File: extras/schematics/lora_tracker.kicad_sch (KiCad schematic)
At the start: 18 parts, among them J1 Conn_Coaxial, J2 Conn_01x10_Female, J3 Conn_01x12_Female, J4 Conn_01x03_Female, U1 ESP32, U2 E22-400M30S, U3 Ai-Thinker-Ra-01

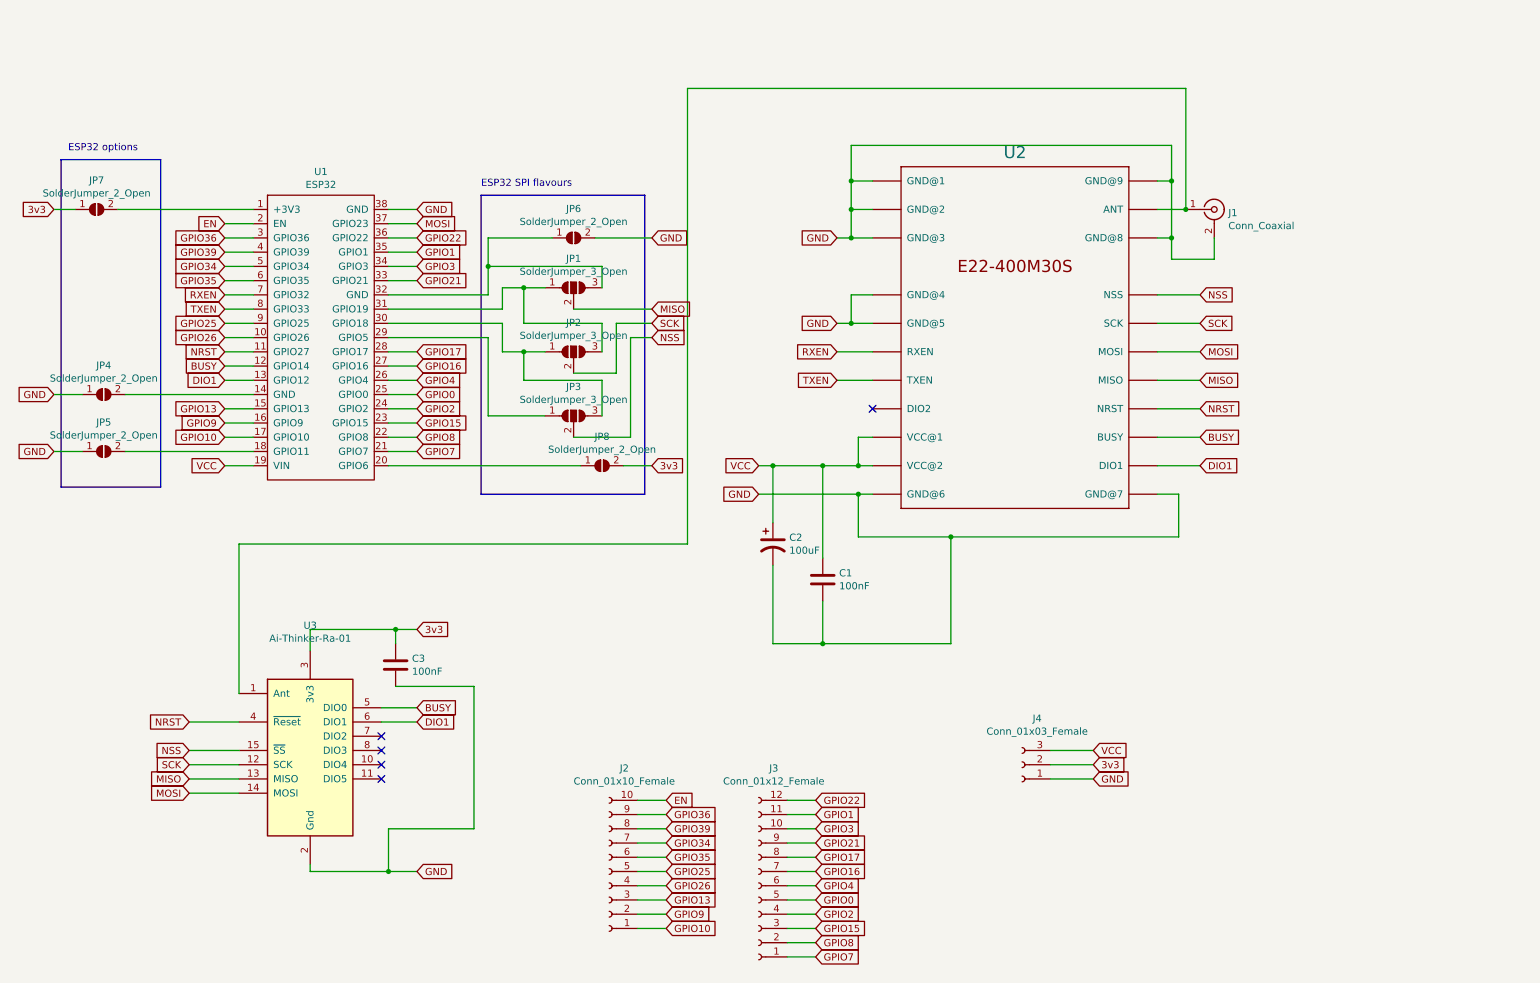
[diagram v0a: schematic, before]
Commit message: Updates
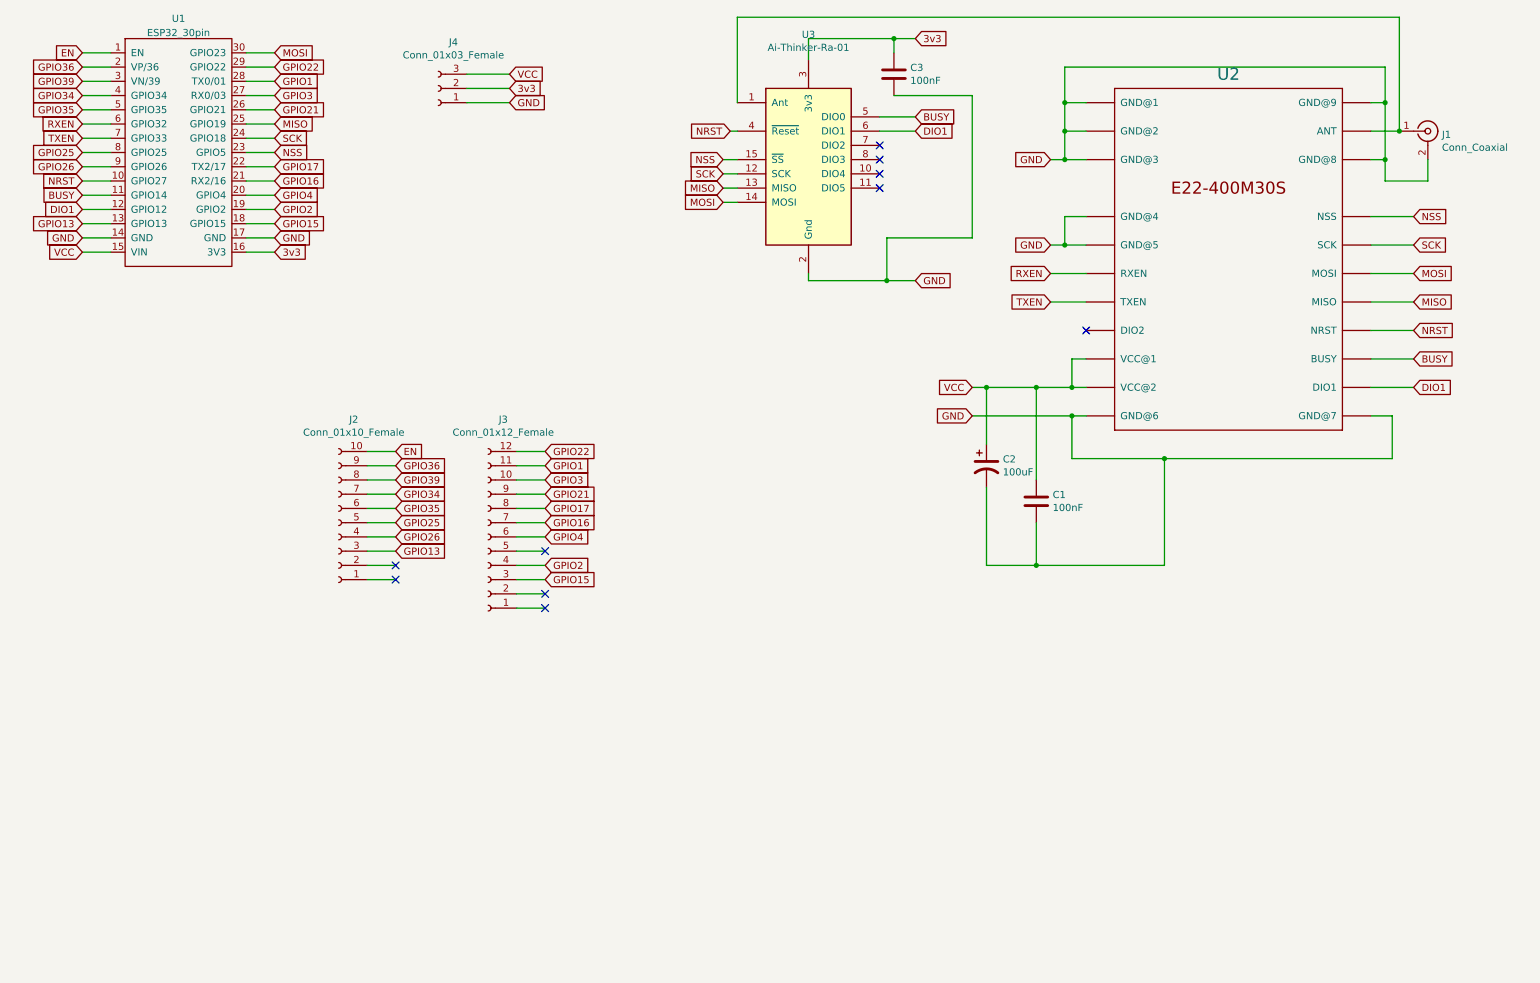
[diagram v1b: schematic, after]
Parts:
- removed JP1, JP2, JP3: SolderJumper_3_Open, Jumper:SolderJumper-3_P1.3mm_Open_Pad1.0x1.5mm, symbol lora_tracker-rescue:SolderJumper_3_Open-Jumper
- removed JP4, JP5, JP6, JP7, JP8: SolderJumper_2_Open, Jumper:SolderJumper-2_P1.3mm_Open_Pad1.0x1.5mm, symbol Jumper:SolderJumper_2_Open
- removed U1: ESP32, lora_tracker:esp32-devkit-wide, symbol lora_tracker:ESP32
- added U1: ESP32_30pin, lora_tracker:esp32-devkit-wide_copy, symbol lora_tracker:ESP32_30pin
- C1, C3: footprint Capacitor_SMD:C_0603_1608Metric_Pad1.05x0.95mm_HandSolder -> Capacitor_SMD:C_0603_1608Metric_Pad1.08x0.95mm_HandSolder
- J1: footprint Connector_Coaxial:SMA_Samtec_SMA-J-P-H-ST-EM1_EdgeMount -> Connector_Coaxial:SMA_Samtec_SMA-J-P-X-ST-EM1_EdgeMount
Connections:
- net 3v3: now also U1.16 (3V3)
- net BUSY: now also U1.11 (GPIO14)
- net DIO1: now also U1.12 (GPIO12)
- net EN: now also U1.1 (EN)
- net GND: now also U1.14 (GND), U1.17 (GND)
- net GPIO1: now also U1.28 (TX0/01)
- net GPIO13: now also U1.13 (GPIO13)
- net GPIO15: now also U1.18 (GPIO15)
- net GPIO16: now also U1.21 (RX2/16)
- net GPIO17: now also U1.22 (TX2/17)
- net GPIO2: now also U1.19 (GPIO2)
- net GPIO21: now also U1.26 (GPIO21)
- net GPIO22: now also U1.29 (GPIO22)
- net GPIO25: now also U1.8 (GPIO25)
- net GPIO26: now also U1.9 (GPIO26)
- net GPIO3: now also U1.27 (RX0/03)
- net GPIO34: now also U1.4 (GPIO34)
- net GPIO35: now also U1.5 (GPIO35)
- net GPIO36: now also U1.2 (VP/36)
- net GPIO39: now also U1.3 (VN/39)
- net GPIO4: now also U1.20 (GPIO4)
- net MISO: now also U1.25 (GPIO19)
- net MOSI: now also U1.30 (GPIO23)
- net NRST: now also U1.10 (GPIO27)
- net NSS: now also U1.23 (GPIO5)
- net RXEN: now also U1.6 (GPIO32)
- net SCK: now also U1.24 (GPIO18)
- net TXEN: now also U1.7 (GPIO33)
- net VCC: now also U1.15 (VIN)
- net GPIO0: no longer names the net of J3.5 (Pin_5)
- net GPIO10: no longer names the net of J2.1 (Pin_1)
- net GPIO7: no longer names the net of J3.1 (Pin_1)
- net GPIO8: no longer names the net of J3.2 (Pin_2)
- net GPIO9: no longer names the net of J2.2 (Pin_2)
- no-connect marks 5 -> 10
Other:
- note removed: "ESP32 SPI flavours"
- note removed: "ESP32 options"
- moved on the sheet: C1, C2, C3, J1, J2, J3, J4, U2, U3

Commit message: Update schematics
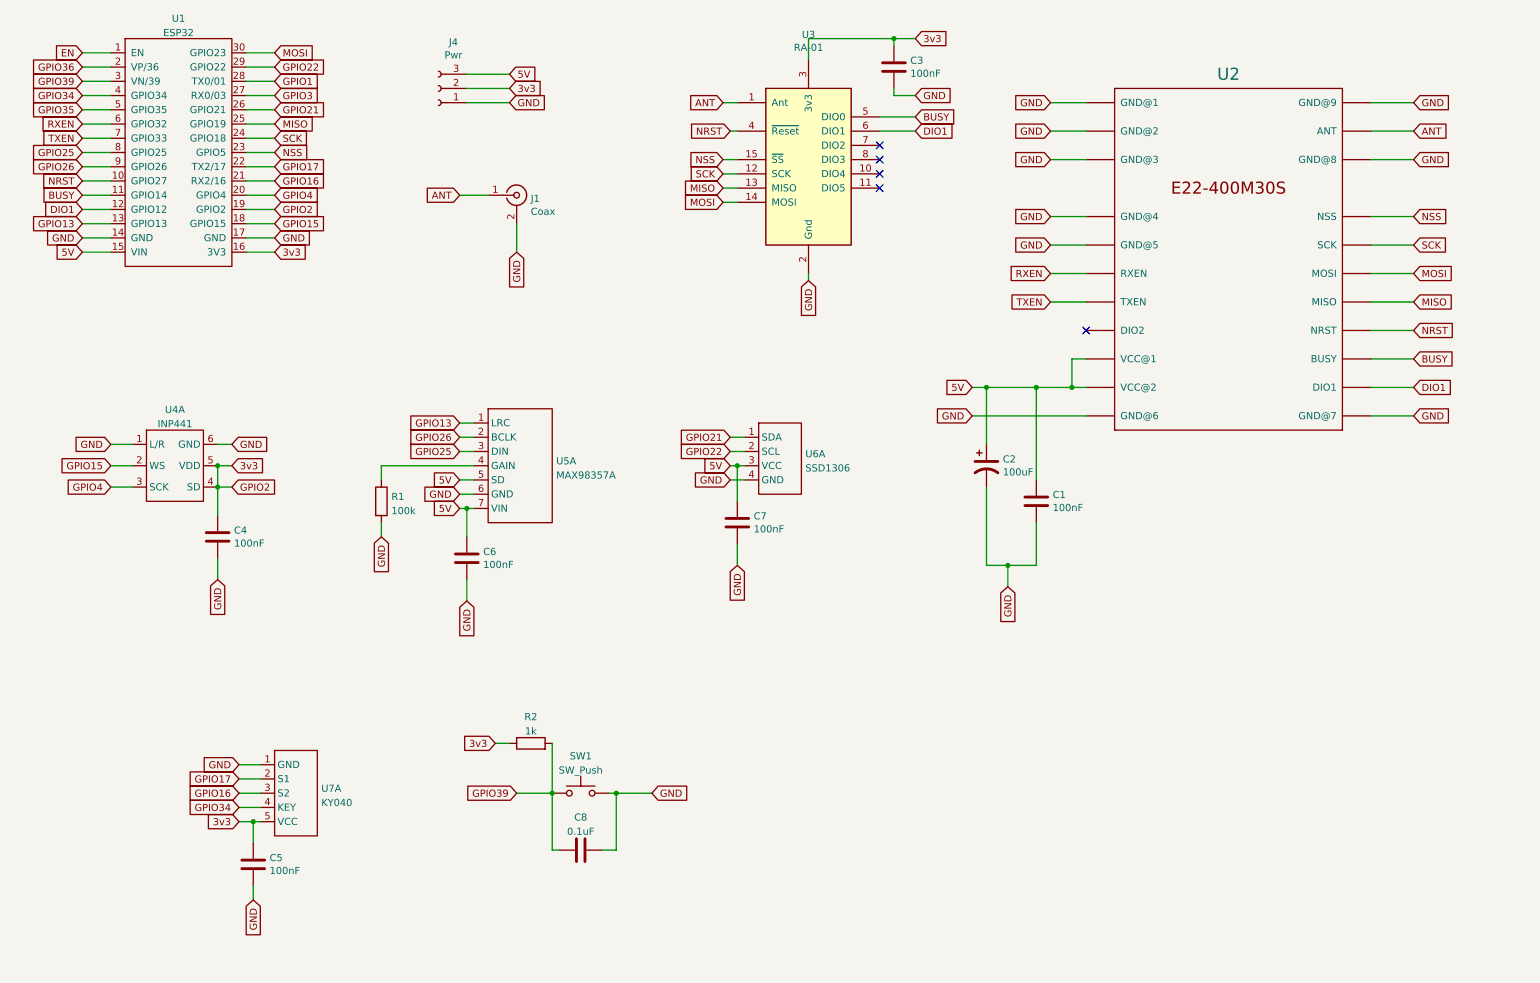
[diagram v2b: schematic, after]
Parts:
- removed J2: Conn_01x10_Female, Connector_PinSocket_2.54mm:PinSocket_1x10_P2.54mm_Vertical, symbol Connector:Conn_01x10_Female
- removed J3: Conn_01x12_Female, Connector_PinSocket_2.54mm:PinSocket_1x12_P2.54mm_Vertical, symbol Connector:Conn_01x12_Female
- added C4, C5, C6, C7: 100nF, Capacitor_SMD:C_0603_1608Metric_Pad1.08x0.95mm_HandSolder, symbol Device:C
- added C8: 0.1uF, symbol Device:C
- added R1: 100k, symbol Device:R
- added R2: 1k, symbol Device:R
- added SW1: SW_Push, symbol Switch:SW_Push
- added U4: INP441, symbol lora_tracker:INP441
- added U5: MAX98357A, symbol lora_tracker:MAX98357A
- added U6: SSD1306, symbol lora_tracker:SSD1306
- added U7: KY040, symbol lora_tracker:KY040
- J1: value Conn_Coaxial -> Coax
- J4: value Conn_01x03_Female -> Pwr
- U1: value ESP32_30pin -> ESP32
- U3: value Ai-Thinker-Ra-01 -> RA-01
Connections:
- net GPIO2 is gone; now on net 3v3: U1.19 (GPIO2)
- net 3v3: now also C4.1, C5.1, R2.1, U4.4 (SD), U4.5 (VDD), U7.5 (VCC)
- net GND: now also C4.2, C5.2, C6.2, C7.2, C8.2, R1.2, SW1.2, U4.1 (L/R), U4.6 (GND), U5.6 (GND), U6.4 (GND), U7.1 (GND)
- net GPIO13: now also U5.1 (LRC)
- net GPIO15: now also U4.2 (WS)
- net GPIO16: now also U7.3 (S2)
- net GPIO17: now also U7.2 (S1)
- net GPIO21: now also U6.1 (SDA)
- net GPIO22: now also U6.2 (SCL)
- net GPIO25: now also U5.3 (DIN)
- net GPIO26: now also U5.2 (BCLK)
- net GPIO34: now also U7.4 (KEY)
- net GPIO39: now also C8.1, R2.2, SW1.1
- net GPIO4: now also U4.3 (SCK)
- net ANT: now reaches J1.1 (In), U2.21 (ANT), U3.1 (Ant)
- net VCC renamed 5V
- net 5V: now also C6.1, C7.1, U5.5 (SD), U5.7 (VIN), U6.3 (VCC)
- new net: R1.1, U5.4 (GAIN)
- no-connect marks 10 -> 5
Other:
- moved on the sheet: C3

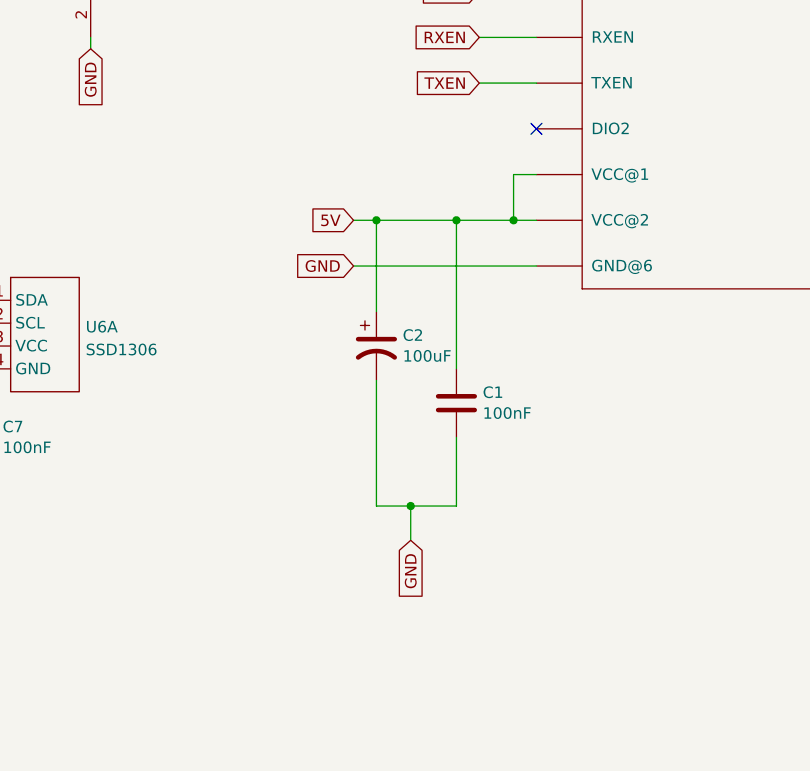
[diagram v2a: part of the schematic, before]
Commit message: Update schematics
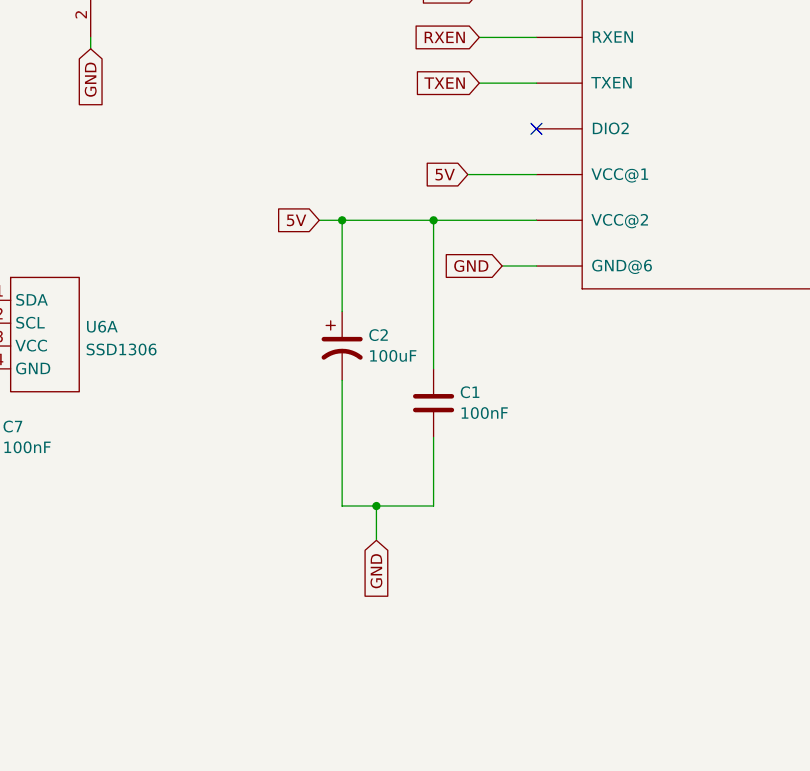
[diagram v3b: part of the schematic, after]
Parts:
- C8: footprint (none) -> Capacitor_SMD:C_0603_1608Metric_Pad1.08x0.95mm_HandSolder
- R1, R2: footprint (none) -> Resistor_SMD:R_0603_1608Metric_Pad0.98x0.95mm_HandSolder
- SW1: footprint (none) -> Button_Switch_THT:SW_Tactile_SKHH_Angled
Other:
- moved on the sheet: C1, C2
